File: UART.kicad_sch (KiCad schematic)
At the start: 3 parts, among them J5 UART1, J6 UART2

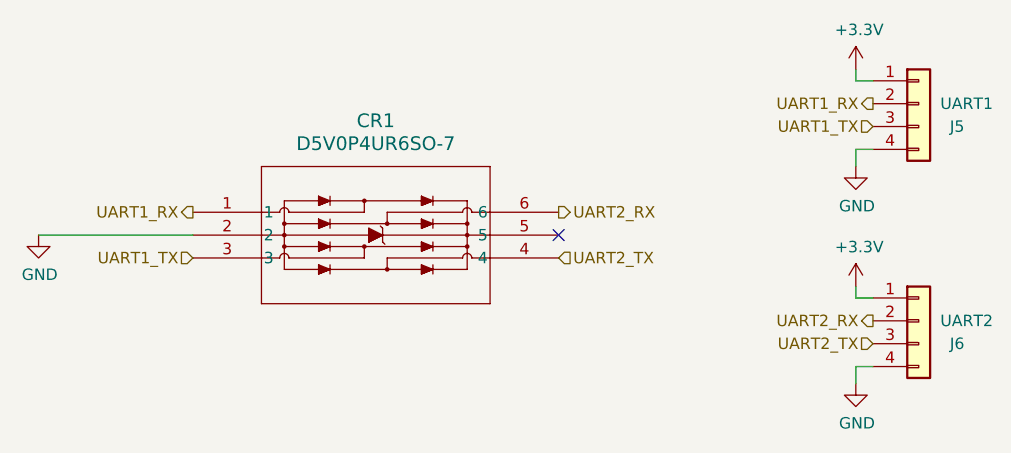
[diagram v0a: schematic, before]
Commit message: Updated pinouts and added protection circuitry for signals
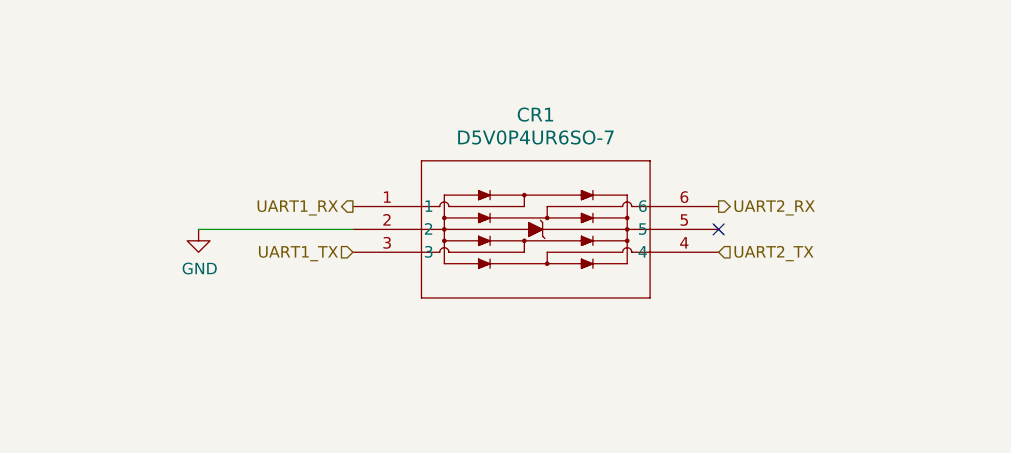
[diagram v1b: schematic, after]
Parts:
- removed J5: UART1, Connector_PinHeader_2.54mm:PinHeader_1x04_P2.54mm_Vertical, symbol Connector_Generic:Conn_01x04
- removed J6: UART2, Connector_PinHeader_2.54mm:PinHeader_1x04_P2.54mm_Vertical, symbol Connector_Generic:Conn_01x04
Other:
- moved on the sheet: CR1
